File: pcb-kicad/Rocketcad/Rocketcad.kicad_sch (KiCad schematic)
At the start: 1 part, among them U1 Teensy4.1

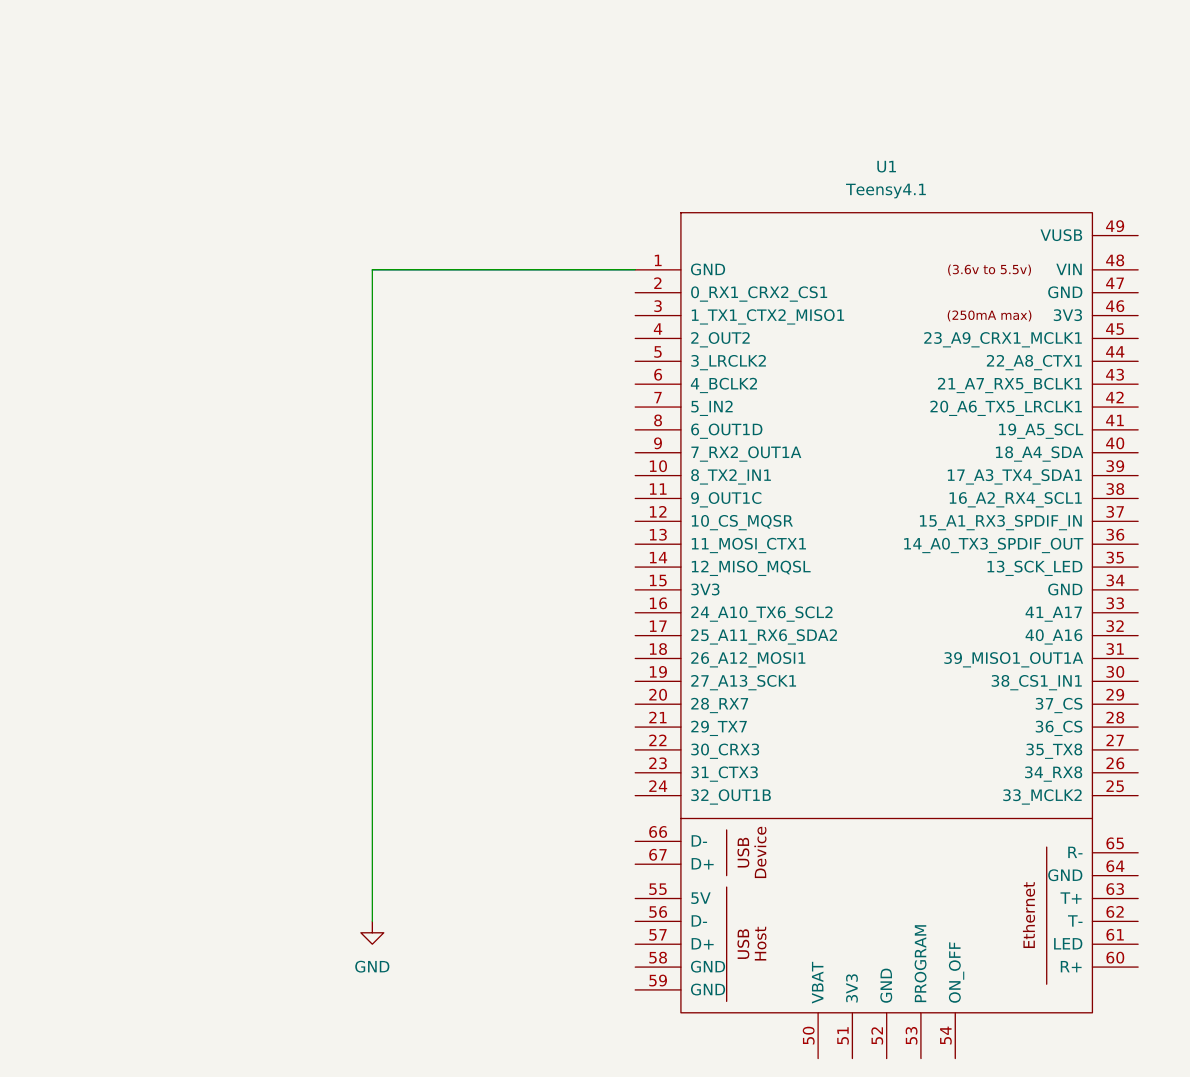
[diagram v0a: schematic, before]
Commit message: structure
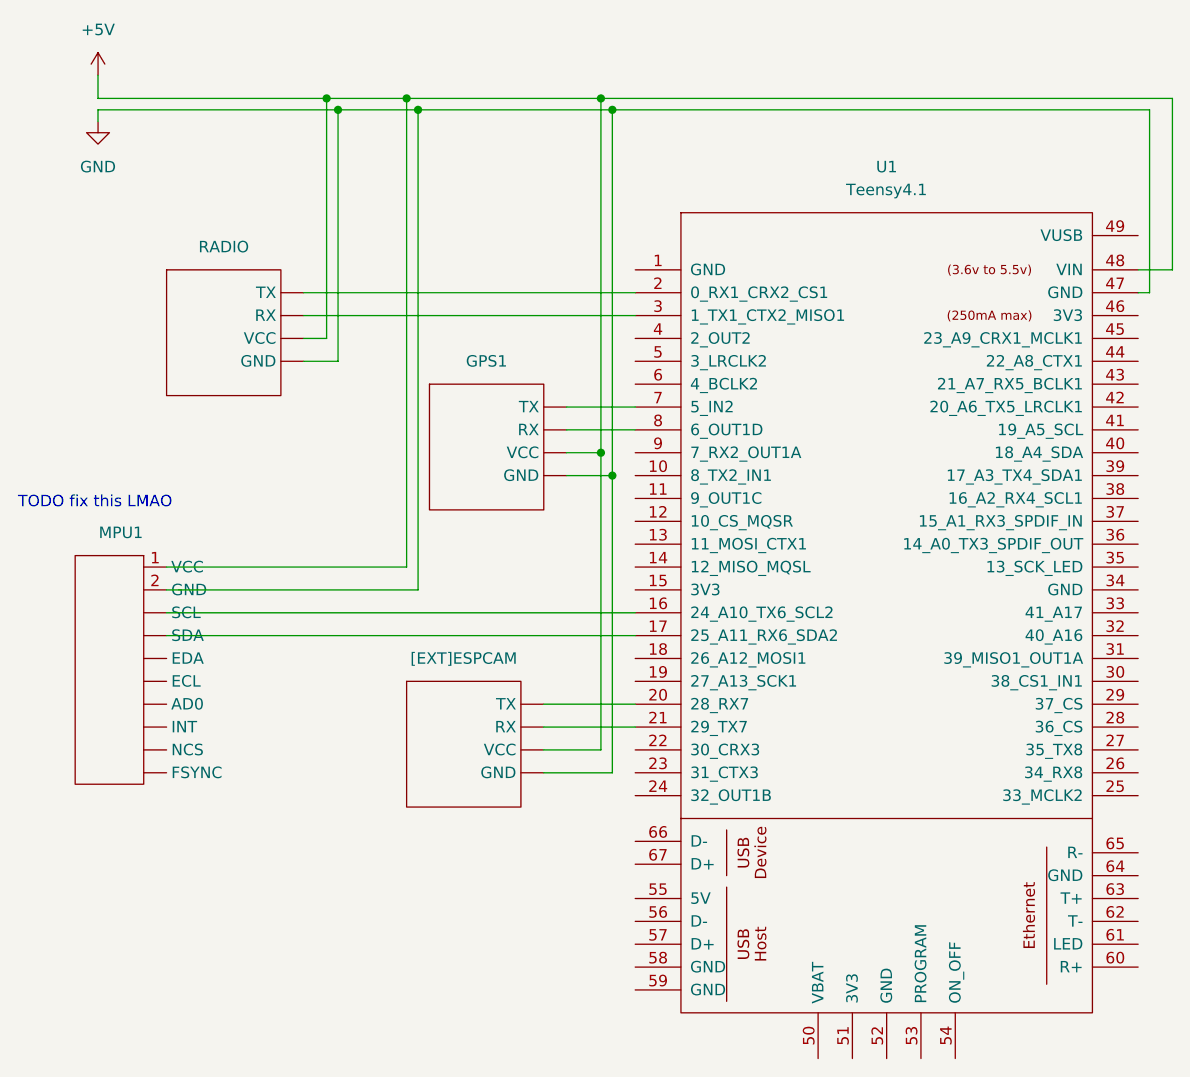
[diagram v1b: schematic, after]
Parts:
- added GPS1, RADIO, [EXT]ESPCAM: ~, symbol New_Library:gps
- added MPU1: ~, symbol New_Library:mpu
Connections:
- net GND: now also U1.47 (GND), GPS1. (VCC), RADIO. (VCC), [EXT]ESPCAM. (VCC); no longer U1.1 (GND)
- net at U1.2 (0_RX1_CRX2_CS1): now also RADIO. (VCC)
- net at U1.20 (28_RX7): now also [EXT]ESPCAM. (VCC)
- net at U1.21 (29_TX7): now also [EXT]ESPCAM. (VCC)
- net at U1.3 (1_TX1_CTX2_MISO1): now also RADIO. (VCC)
- net +5V: now reaches U1.48 (VIN)
- net +5V: now also GPS1. (VCC), RADIO. (VCC), [EXT]ESPCAM. (VCC)
- net at U1.7 (5_IN2): now also GPS1. (VCC)
- net at U1.8 (6_OUT1D): now also GPS1. (VCC)
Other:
- note added: "TODO fix this LMAO"
